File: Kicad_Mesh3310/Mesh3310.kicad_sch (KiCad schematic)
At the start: 16 parts, among them J1 USB device, SW2 "OK"

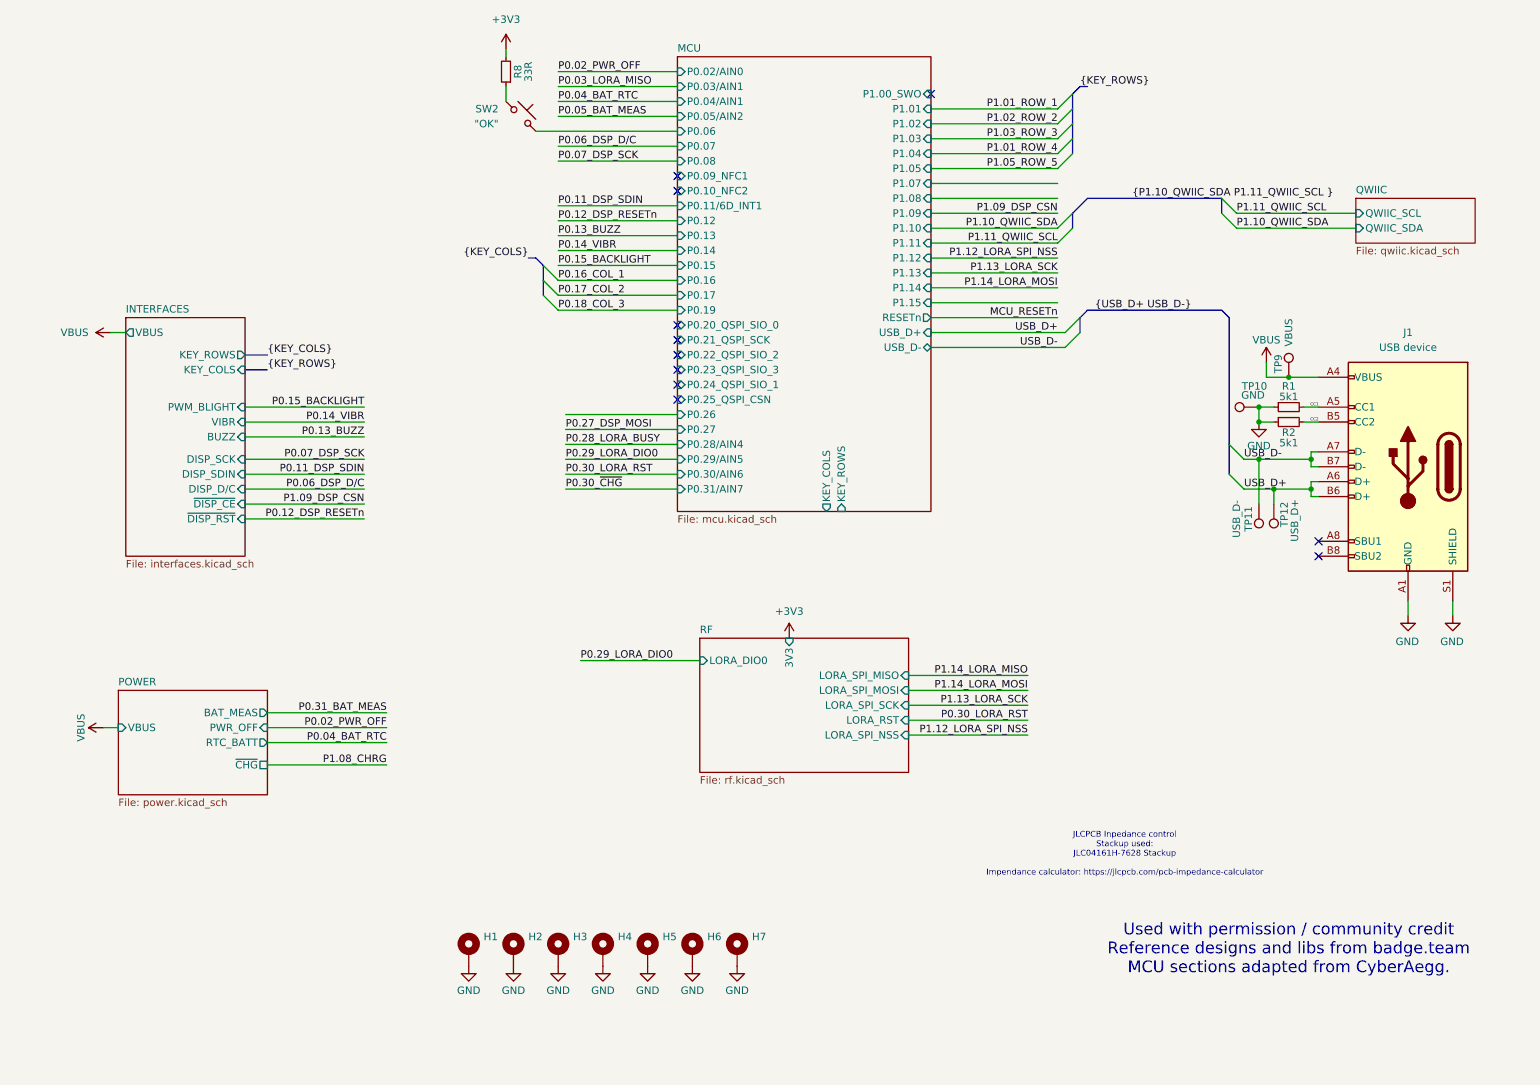
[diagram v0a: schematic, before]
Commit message: cleanup
schematic cleanup
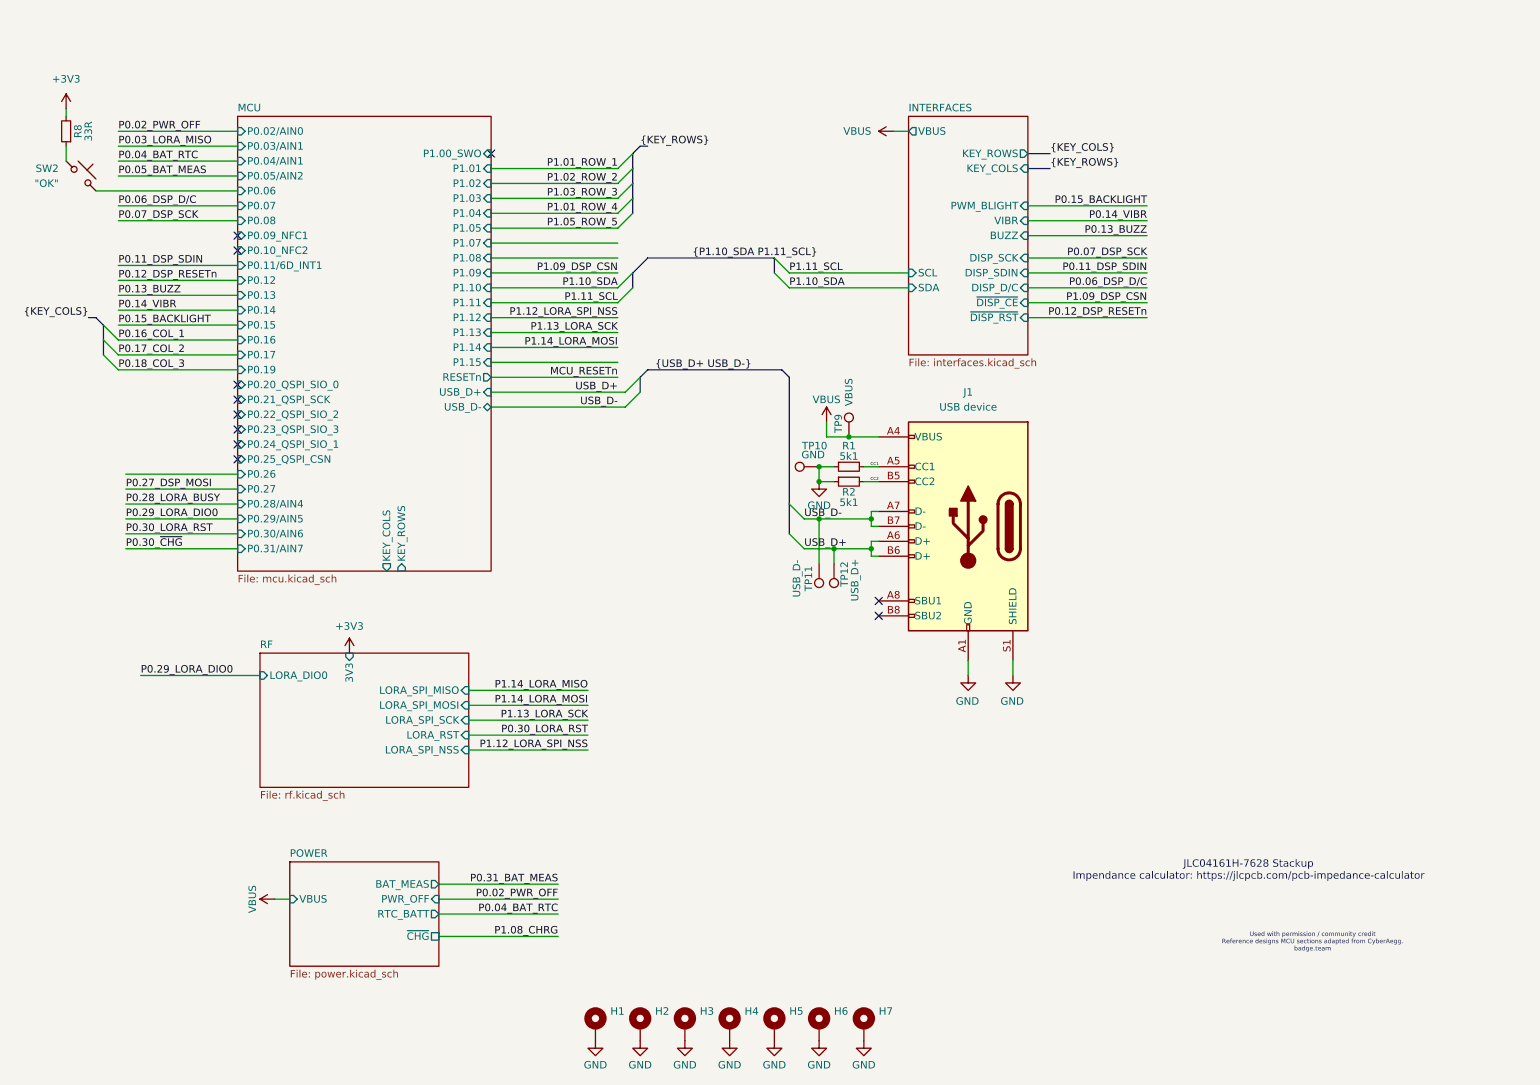
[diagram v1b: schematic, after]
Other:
- removed sheet QWIIC
- sheet INTERFACES ports: added SCL, SDA; removed none
- note added: "JLC04161H-7628 Stackup Impendance calculator: https://jlcpcb.com/pcb-impedance-calculator"
- note added: "Used with permission / community credit Reference designs MCU sections adapted from CyberAegg. badge.team"
- note removed: "JLCPCB Inpedance control Stackup used: JLC04161H-7628 Stackup Impendance calculator: https://jlcpcb.com/pcb-impedance-calculator"
- note removed: "Used with permission / community credit Reference designs and libs from badge.team MCU sections adapted from CyberAegg."
- moved on the sheet: H1, H2, H3, H4, H5, H6, H7, J1, R1, R2, R8, SW2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
